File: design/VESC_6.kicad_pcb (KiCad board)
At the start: 4 copper layers, 60 x 60 mm, 303 parts, among them P1 USB_OTG, P10 PH_C, P11 SUPPLY, P12 GND, P2 BATT_-, P2 CAN, P4 HALL_ENC, P5 COM, P6 SERVO, P7 SWD, P8 PH_A, P9 PH_B, Q1 IRF7749, Q2 IRF7749, Q3 IRF7749, Q4 IRF7749, Q5 IRF7749, Q6 IRF7749, U1 STM32F40X_LQFP64, U10 MPU9150, U11 SENSOR_VOLTAGE, U2 LM3671, U3 DRV8301, U4 TJA1051TK3, U5 AD8418, U6 AD8418, U7 AD8418, U8 NRF24L01P, U9 CONN_U_FL, X1 8m, X2 16M

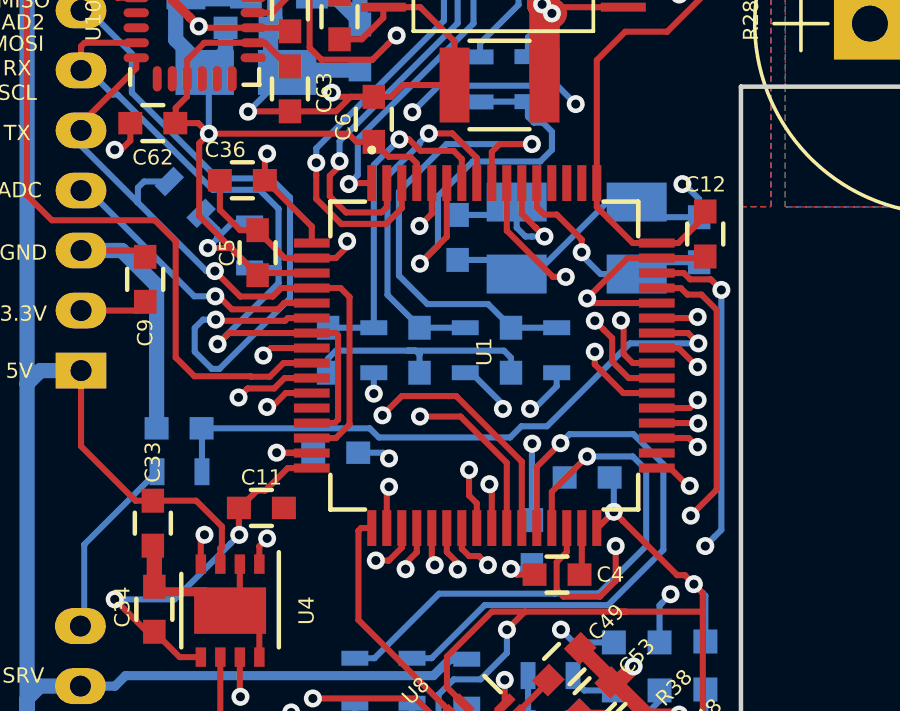
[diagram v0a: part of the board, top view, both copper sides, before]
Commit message: initial commit
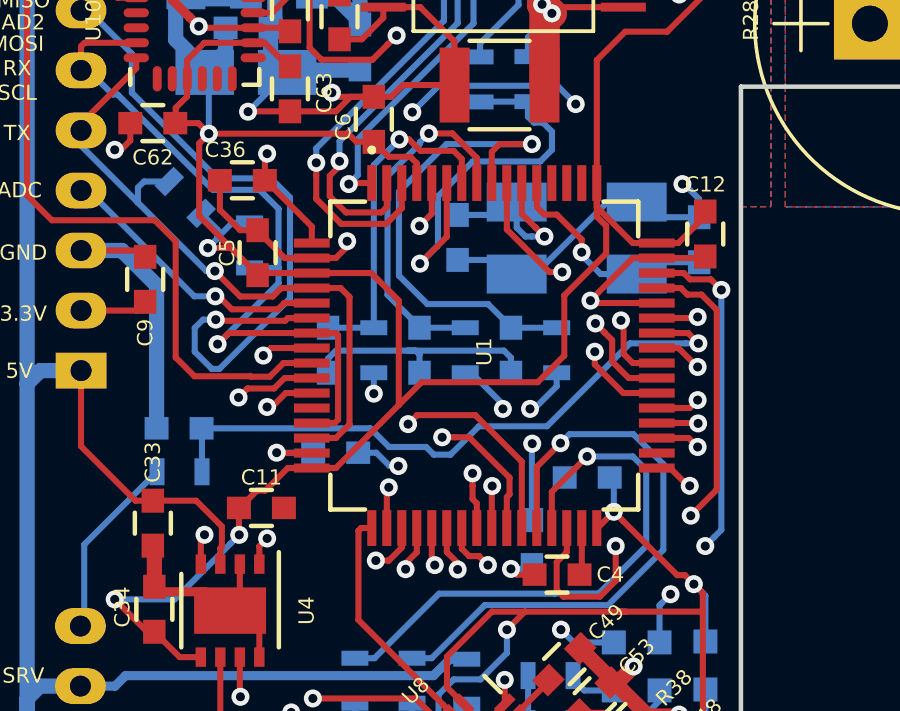
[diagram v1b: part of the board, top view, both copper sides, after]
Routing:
- net VCC: track 202.0 -> 225.2 mm
- net /MCU/H3: track 27.1 -> 26.2 mm
- net /MCU/H2: track 26.1 -> 25.4 mm
- net /DRV8301/INL_A: track 25.6 -> 26.3 mm
